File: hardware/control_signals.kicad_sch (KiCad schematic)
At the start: 25 parts, among them Q10 BC557, Q11 BC557, Q12 BC547, Q9 BC557, U8 74LS06N

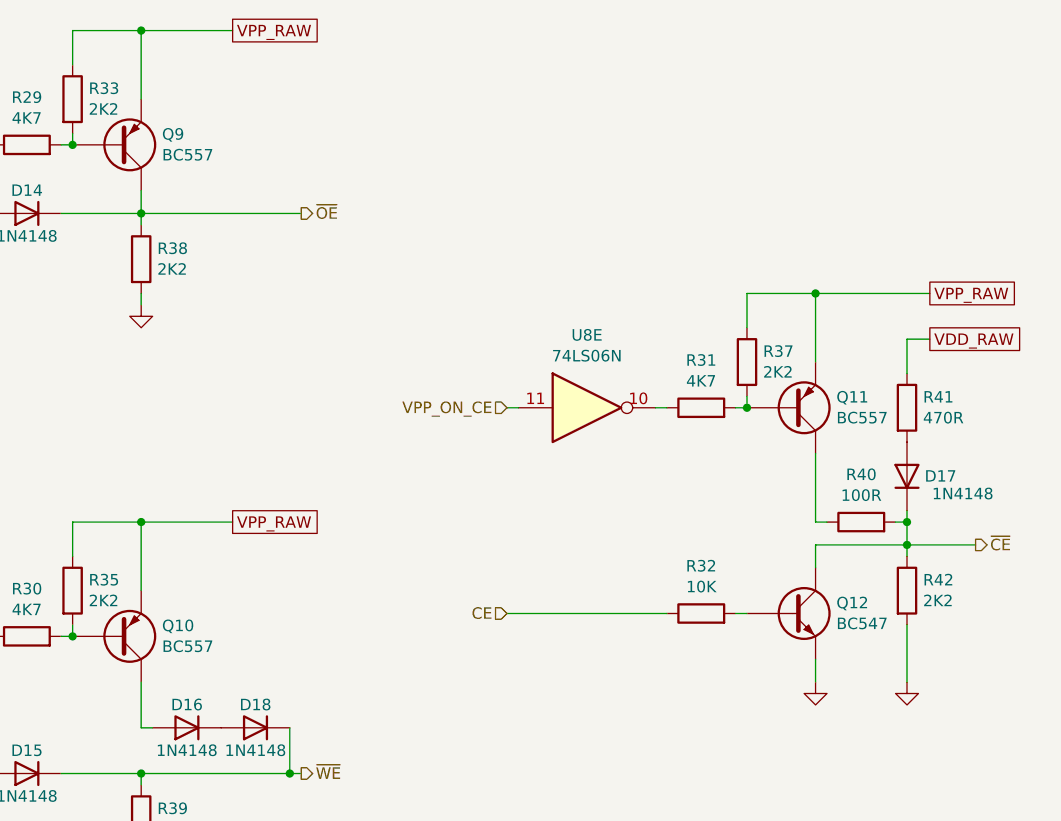
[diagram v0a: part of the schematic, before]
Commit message: Rev.E. Updated specifications document and hardware design.
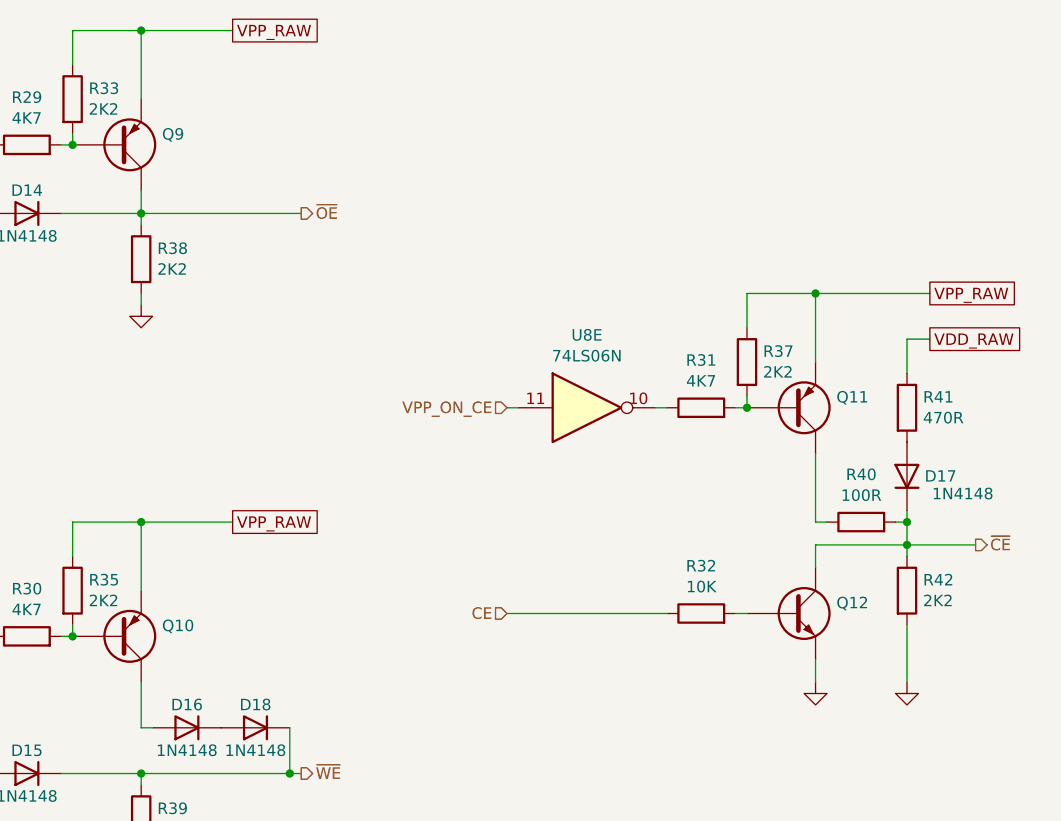
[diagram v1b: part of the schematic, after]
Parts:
- Q10, Q11, Q9: value BC557 -> (none); footprint Package_TO_SOT_THT:TO-92_Inline_Wide -> (none)
- Q12: value BC547 -> (none); footprint Package_TO_SOT_THT:TO-92_Inline_Wide -> (none)
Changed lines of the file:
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@@
       (effects (font (size 1.27 1.27)) (justify left))
     )
-    (property "Value" "BC557" (id 1) (at 149.6314 49.403 0)
-      (effects (font (size 1.27 1.27)) (justify left))
-    )
-    (property "Footprint" "Package_TO_SOT_THT:TO-92_Inline_Wide" (id 2) (at 149.86 46.355 0)
+    (property "Value" "" (id 1) (at 149.6314 49.403 0)
+      (effects (font (size 1.27 1.27)) (justify left))
+    )
+    (property "Footprint" "" (id 2) (at 149.86 46.355 0)
       (effects (font (size 1.27 1.27) italic) (justify left) hide)
     )
@@
       (effects (font (size 1.27 1.27)) (justify left))
     )
-    (property "Value" "BC557" (id 1) (at 149.6314 104.013 0)
-      (effects (font (size 1.27 1.27)) (justify left))
-    )
-    (property "Footprint" "Package_TO_SOT_THT:TO-92_Inline_Wide" (id 2) (at 149.86 100.965 0)
+    (property "Value" "" (id 1) (at 149.6314 104.013 0)
+      (effects (font (size 1.27 1.27)) (justify left))
+    )
+    (property "Footprint" "" (id 2) (at 149.86 100.965 0)
       (effects (font (size 1.27 1.27) italic) (justify left) hide)
     )
@@
       (effects (font (size 1.27 1.27)) (justify left))
     )
-    (property "Value" "BC557" (id 1) (at 224.5614 78.613 0)
-      (effects (font (size 1.27 1.27)) (justify left))
-    )
-    (property "Footprint" "Package_TO_SOT_THT:TO-92_Inline_Wide" (id 2) (at 224.79 75.565 0)
+    (property "Value" "" (id 1) (at 224.5614 78.613 0)
+      (effects (font (size 1.27 1.27)) (justify left))
+    )
+    (property "Footprint" "" (id 2) (at 224.79 75.565 0)
       (effects (font (size 1.27 1.27) italic) (justify left) hide)
     )
@@
       (effects (font (size 1.27 1.27)) (justify left))
     )
-    (property "Value" "BC547" (id 1) (at 224.5614 101.473 0)
-      (effects (font (size 1.27 1.27)) (justify left))
-    )
-    (property "Footprint" "Package_TO_SOT_THT:TO-92_Inline_Wide" (id 2) (at 224.79 102.235 0)
+    (property "Value" "" (id 1) (at 224.5614 101.473 0)
+      (effects (font (size 1.27 1.27)) (justify left))
+    )
+    (property "Footprint" "" (id 2) (at 224.79 102.235 0)
       (effects (font (size 1.27 1.27) italic) (justify left) hide)
     )
